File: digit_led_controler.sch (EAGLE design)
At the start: 37 parts

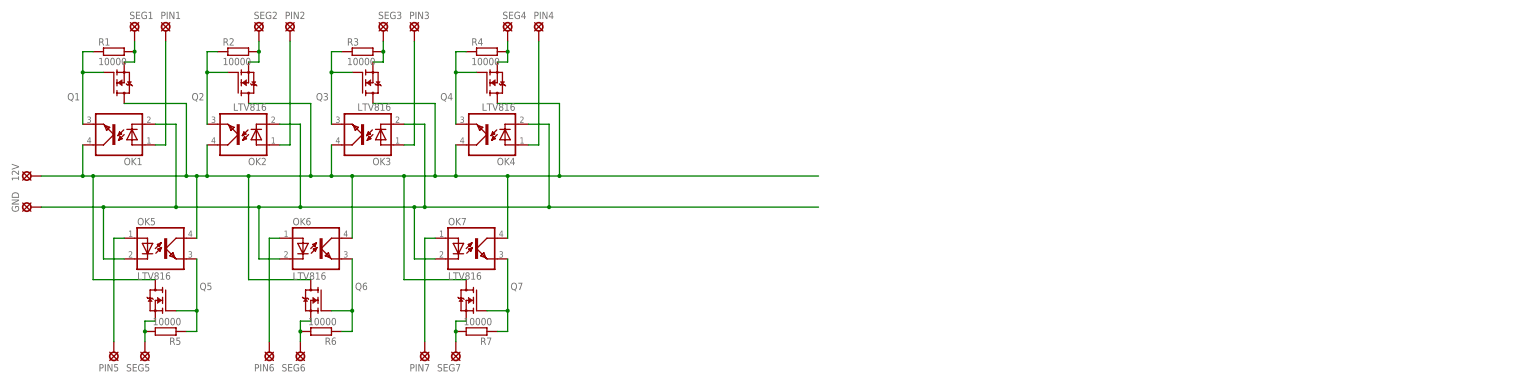
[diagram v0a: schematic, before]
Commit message: Update digit_led_controler.sch
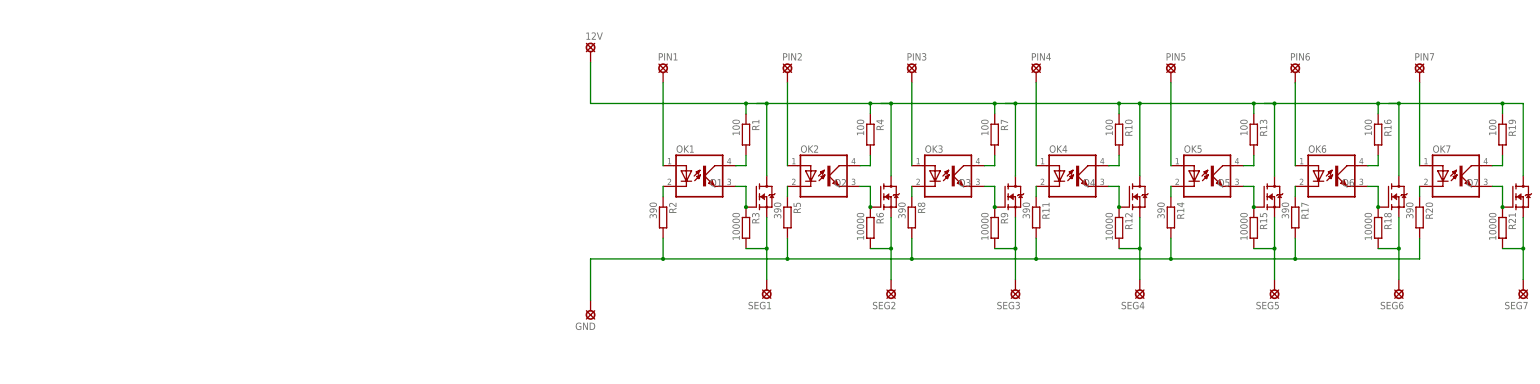
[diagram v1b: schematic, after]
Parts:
- added R10, R13, R16, R19: 100, resistor:R-EU_R0805
- added R11, R14, R17, R20, R8: 390, resistor:R-EU_R0805
- added R12, R15, R18, R21, R9: 10000, resistor:R-EU_R0805
- R1, R4, R7: value 10000 -> 100; device resistor:R-EU_R1206 -> resistor:R-EU_R0805
- R2, R5: value 10000 -> 390; device resistor:R-EU_R1206 -> resistor:R-EU_R0805
- R3, R6: device resistor:R-EU_R1206 -> resistor:R-EU_R0805
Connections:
- removed net 12V: 12V.MP, OK1.COL, OK2.COL, OK3.COL, OK4.COL, OK5.COL, OK6.COL, OK7.COL, Q1.D, Q2.D, Q3.D, Q4.D, Q5.D, Q6.D, Q7.D
- removed net GND: GND.MP, OK1.C, OK2.C, OK3.C, OK4.C, OK5.C, OK6.C, OK7.C
- removed net N$13 (its old number): OK5.EMIT, Q5.G, R5.1
- removed net N$14: Q5.S, R5.2, SEG5.MP
- removed net N$19 (its old number): OK7.EMIT, Q7.G, R7.1
- removed net N$20: Q7.S, R7.2, SEG7.MP
- removed net N$5: Q2.S, R2.2, SEG2.MP
- removed net N$7: OK3.EMIT, Q3.G, R3.1
- new net N$12: Q2.S, R6.2, SEG2.MP
- new net N$15: OK4.COL, R10.2
- new net N$18: Q3.S, R9.2, SEG3.MP
- new net N$21: OK5.COL, R13.2
- new net N$22: OK4.EMIT, Q4.G, R12.1
- new net N$23: OK6.COL, R16.2
- new net N$24: Q4.S, R12.2, SEG4.MP
- new net N$27: OK1.C, R2.1
- new net N$28: OK5.EMIT, Q5.G, R15.1
- new net N$29: OK2.C, R5.1
- new net N$30: Q5.S, R15.2, SEG5.MP
- new net N$33: OK3.C, R8.1
- new net N$34: OK6.EMIT, Q6.G, R18.1
- new net N$35: OK4.C, R11.1
- new net N$36: Q6.S, R18.2, SEG6.MP
- new net N$39: OK5.C, R14.1
- new net N$4: Q1.S, R3.2, SEG1.MP
- new net N$40: OK7.EMIT, Q7.G, R21.1
- new net N$41: OK6.C, R17.1
- new net N$42: Q7.S, R21.2, SEG7.MP
- new net N$44: OK7.C, R20.1
- new net N$9: GND.MP, R11.2, R14.2, R17.2, R2.2, R20.2, R5.2, R8.2
- net N$1: now also 12V.MP, Q1.D, Q2.D, Q3.D, Q4.D, Q5.D, Q6.D, Q7.D, R10.1, R13.1, R16.1, R19.1, R4.1, R7.1; no longer OK1.EMIT, Q1.G
- net N$10: now also OK2.EMIT, Q2.G, R6.1; no longer OK4.EMIT, Q4.G, R4.1
- net N$11: now also OK3.COL, R7.2; no longer Q4.S, R4.2, SEG4.MP
- net N$16: now also OK3.EMIT, Q3.G, R9.1; no longer OK6.EMIT, Q6.G, R6.1
- net N$17: now also OK7.COL, R19.2; no longer Q6.S, R6.2, SEG6.MP
- net N$2: now also OK1.EMIT, Q1.G, R3.1; no longer OK2.EMIT, Q2.G, R2.1
- net N$3: now also OK2.COL, R4.2; no longer Q1.S, R1.2, SEG1.MP
- net N$8: now also OK1.COL, R1.2; no longer Q3.S, R3.2, SEG3.MP
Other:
- moved on the sheet: 12V, GND, OK1, OK2, OK3, OK4, OK5, OK6, OK7, PIN1, PIN2, PIN3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

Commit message: Update digit_led_controler.sch
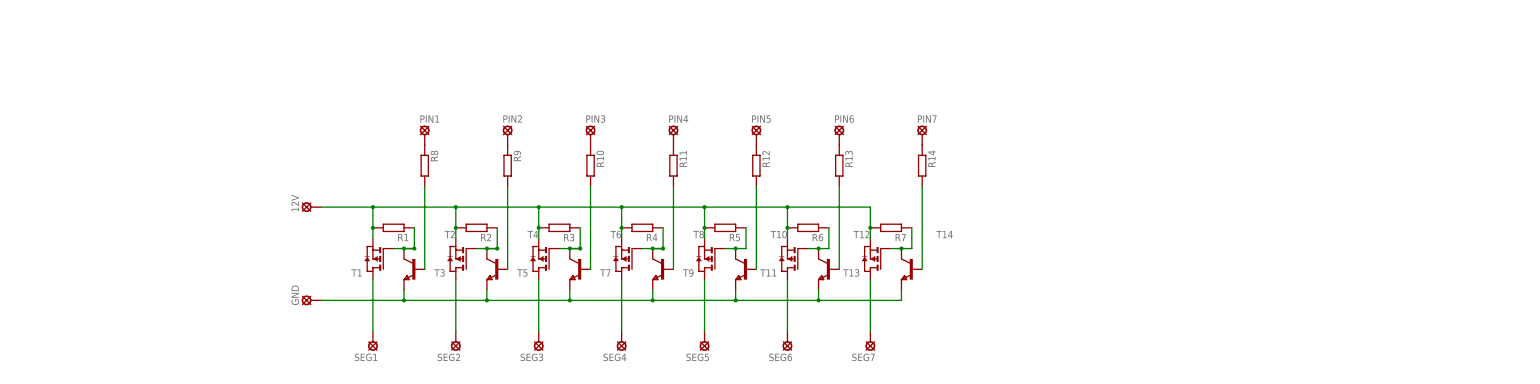
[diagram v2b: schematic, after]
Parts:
- removed OK1, OK2, OK3, OK4, OK5, OK6, OK7: LTV816, optocoupler:LTV816
- removed Q1, Q2, Q3, Q4, Q5, Q6, Q7: (no value), myMOSFET:IRFML8244
- removed R15, R18, R21: 10000, resistor:R-EU_R0805
- removed R16, R19: 100, resistor:R-EU_R0805
- removed R17, R20: 390, resistor:R-EU_R0805
- added T1, T11, T13, T3, T5, T7, T9: (no value), zetex:PMOSSOT23
- added T10, T12, T14, T2, T4, T6, T8: (no value), zetex:NPNSOT23
- 12V, GND, PIN1, PIN2, PIN3, PIN4, PIN5, PIN6, PIN7, SEG1, SEG2, SEG3, SEG4, SEG5, SEG6, SEG7: value LSP13 -> SE14; device solpad:LSP13 -> solpad:SE14
- R1, R10, R13, R4, R7: value 100 -> (none)
- R11, R14, R2, R5, R8: value 390 -> (none)
- R12, R3, R6, R9: value 10000 -> (none)
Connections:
- removed net N$24: Q4.S, R12.2, SEG4.MP
- removed net N$25: OK4.A, PIN4.MP
- removed net N$27: OK1.C, R2.1
- removed net N$28: OK5.EMIT, Q5.G, R15.1
- removed net N$29: OK2.C, R5.1
- removed net N$30: Q5.S, R15.2, SEG5.MP
- removed net N$31: OK5.A, PIN5.MP
- removed net N$34: OK6.EMIT, Q6.G, R18.1
- removed net N$35: OK4.C, R11.1
- removed net N$36: Q6.S, R18.2, SEG6.MP
- removed net N$39: OK5.C, R14.1
- removed net N$40: OK7.EMIT, Q7.G, R21.1
- removed net N$41: OK6.C, R17.1
- removed net N$42: Q7.S, R21.2, SEG7.MP
- removed net N$43: OK7.A, PIN7.MP
- removed net N$44: OK7.C, R20.1
- new net N$14: PIN7.MP, R14.1
- new net N$20: R12.2, T10.B
- new net N$26: SEG4.MP, T7.D
- new net N$46: R6.1, T11.G, T12.C
- new net N$5: R2.1, T3.G, T4.C
- new net N$50: SEG6.MP, T11.D
- new net N$61: R7.1, T13.G, T14.C
- new net N$65: SEG7.MP, T13.D
- new net N$7: PIN2.MP, R9.1
- net N$1: now also PIN1.MP, R8.1; no longer 12V.MP, Q1.D, Q2.D, Q3.D, Q4.D, Q5.D, Q6.D, Q7.D, R1.1, R10.1, R13.1, R16.1, R19.1, R4.1, R7.1
- net N$10: now also SEG2.MP, T3.D; no longer OK2.EMIT, Q2.G, R6.1
- net N$11: now also PIN5.MP, R12.1; no longer OK3.COL, R7.2
- net N$12: now also PIN6.MP, R13.1; no longer Q2.S, R6.2, SEG2.MP
- net N$13: now also R3.1, T5.G, T6.C; no longer OK2.A, PIN2.MP
- net N$15: now also R8.2, T2.B; no longer OK4.COL, R10.2
- net N$16: now also R9.2, T4.B; no longer OK3.EMIT, Q3.G, R9.1
- net N$17: now also SEG3.MP, T5.D; no longer OK7.COL, R19.2
- net N$18: now also R10.2, T6.B; no longer Q3.S, R9.2, SEG3.MP
- net N$19: now also R11.2, T8.B; no longer OK3.A, PIN3.MP
- net N$2: now also R1.1, T1.G, T2.C; no longer OK1.EMIT, Q1.G, R3.1
- net N$21: now also T12.B; no longer OK5.COL
- net N$22: now also R4.1, T7.G, T8.C; no longer OK4.EMIT, Q4.G, R12.1
- net N$23: now also R14.2, T14.B; no longer OK6.COL, R16.2
- net N$3: now also GND.MP, T10.E, T12.E, T14.E, T2.E, T4.E, T6.E, T8.E; no longer OK2.COL, R4.2
- net N$33: now also R5.1, T10.C, T9.G; no longer OK3.C, R8.1
- net N$37: now also SEG5.MP, T9.D; no longer OK6.A, PIN6.MP
- net N$4: now also T1.D; no longer Q1.S, R3.2
- net N$6: now also 12V.MP, R1.2, R2.2, R3.2, R4.2, R5.2, R6.2, R7.2, T1.S, T11.S, T13.S, T3.S, T5.S, T7.S, T9.S; no longer OK1.A, PIN1.MP
- net N$8: now also PIN3.MP, R10.1; no longer OK1.COL, R1.2
- net N$9: now also PIN4.MP, R11.1; no longer GND.MP, R11.2, R14.2, R17.2, R2.2, R20.2, R5.2, R8.2
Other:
- moved on the sheet: 12V, GND, PIN1, PIN2, PIN3, PIN4, PIN5, PIN6, PIN7, R1, R10, R11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
